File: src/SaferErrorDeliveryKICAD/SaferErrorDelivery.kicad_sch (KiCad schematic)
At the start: 4 parts, among them U1 74HC04, U2 74LS21, U3 74LS11, U4 4072

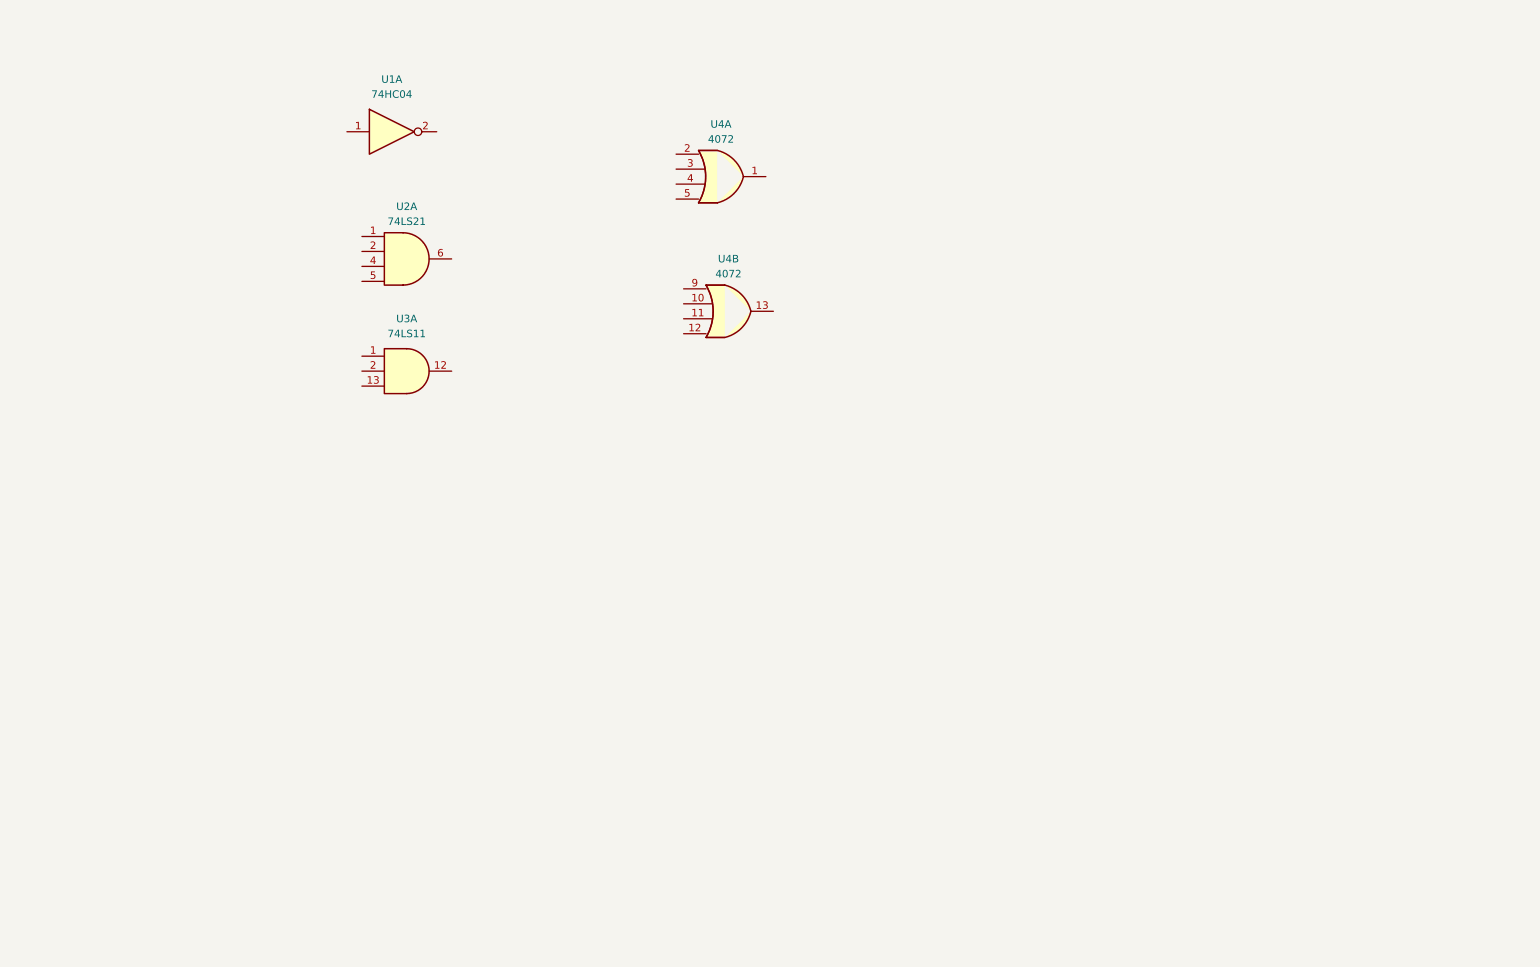
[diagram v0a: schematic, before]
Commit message: Updated kiCAD wiring
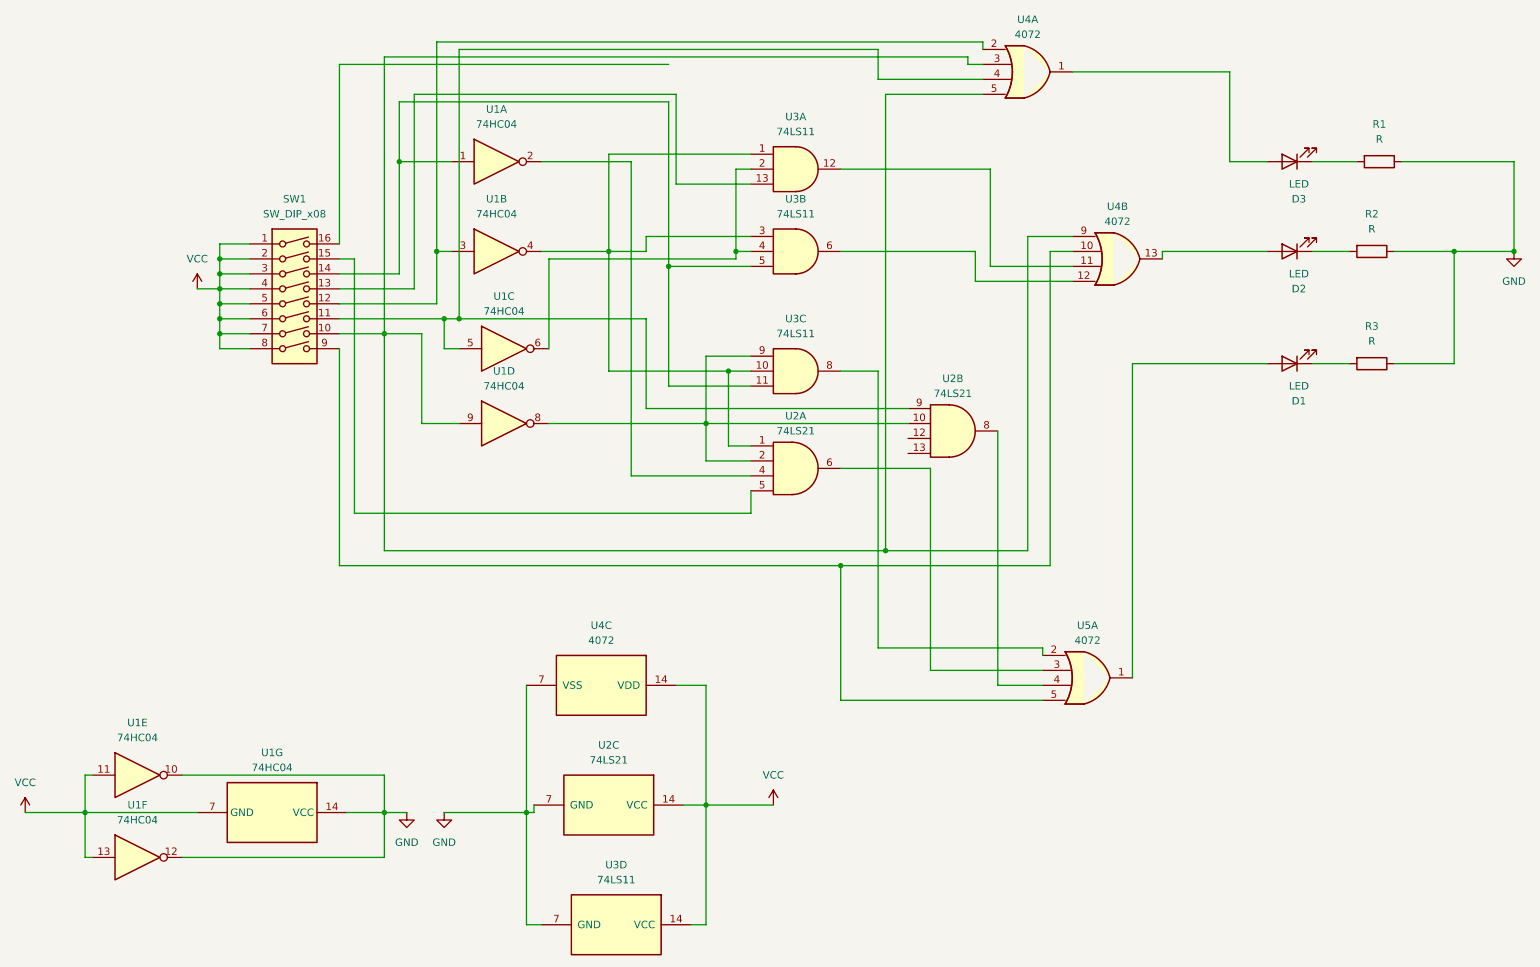
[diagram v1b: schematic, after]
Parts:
- added D1, D2, D3: LED, symbol Device:LED
- added R1, R2, R3: R, symbol Device:R
- added SW1: SW_DIP_x08, symbol Switch:SW_DIP_x08
- added unit 4 of U1
- added unit 5 of U1
- added unit 6 of U1
- added unit 7 of U1
- added unit 2 of U1
- added unit 3 of U1
- added unit 3 of U2
- added unit 2 of U2
- added unit 4 of U3
- added unit 2 of U3
- added unit 3 of U3
- added unit 3 of U4
- added U5: 4072, symbol 4xxx:4072
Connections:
- net at U4.10: now also SW1.9, U5.5
- net at U4.11: now also U3.12
- net at U4.12: now also U3.6
- net at U4.13: now also D2.2 (A)
- net at U4.9: now also U4.3, U4.5, SW1.10, U1.9
- net at U1.1: now also SW1.14, U3.11, U3.5
- net at U1.2: now also U2.4
- net at U4.1: now also D3.2 (A)
- net at U4.2: now also SW1.12, U1.3
- net at U4.4: now also SW1.11, U1.5, U2.9
- net at U2.1: now also U3.1, U1.4, U3.10, U3.3
- net at U2.2: now also U1.8, U2.10, U3.9
- net at U2.5: now also SW1.15
- net at U2.6: now also U5.3
- net at U3.13: now also SW1.13
- net at U3.2: now also U1.6, U3.4
- new net: D1.1 (K), R3.2
- new net: D2.1 (K), R2.2
- new net: U3.8, U5.2
- new net: D1.2 (A), U5.1
- new net: U2.8, U5.4
- new net: D3.1 (K), R1.2
- new net GND: R1.1, R2.1, R3.1, U1.10, U1.12, U1.14 (VCC), U2.7 (GND), U3.7 (GND), U4.7 (VSS)
- new net VCC: SW1.1, SW1.2, SW1.3, SW1.4, SW1.5, SW1.6, SW1.7, SW1.8, U1.11, U1.13, U1.7 (GND), U2.14 (VCC), U3.14 (VCC), U4.14 (VDD)
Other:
- moved on the sheet: U1A, U2A, U3A, U4A, U4B
